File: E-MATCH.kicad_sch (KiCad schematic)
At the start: 7 parts, among them IC1 NCV81071BZR2G, J2 691137710002, Q1 IRF3205, U1 TMCS1108A2UQDR

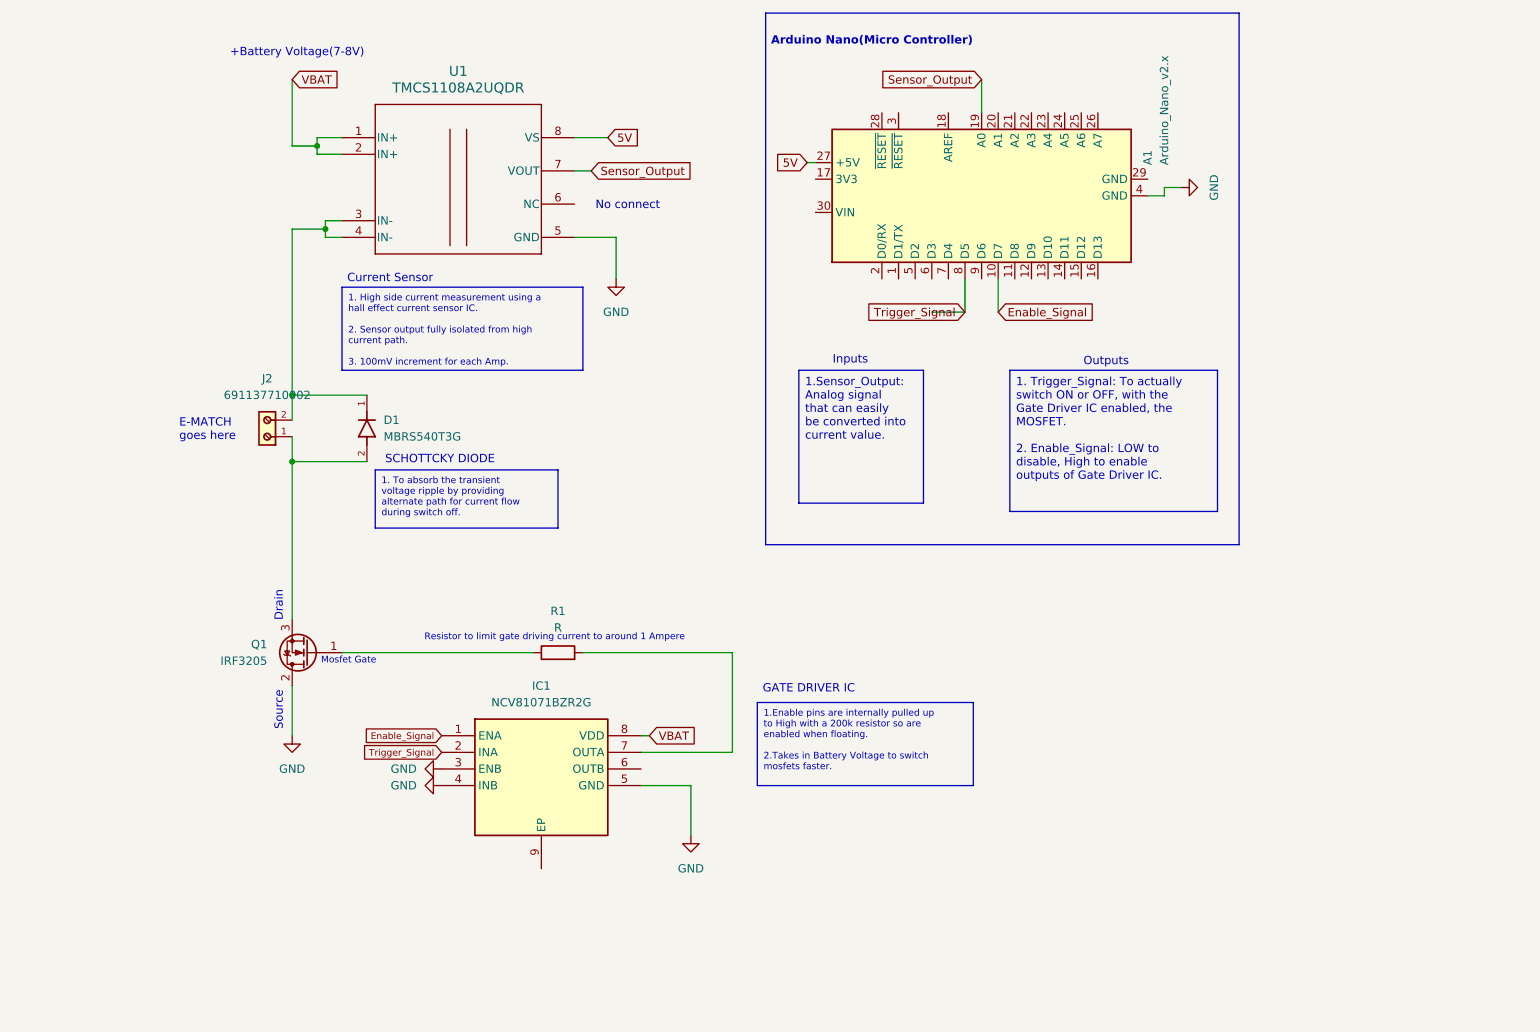
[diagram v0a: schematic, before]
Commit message: Neat placement for schematic
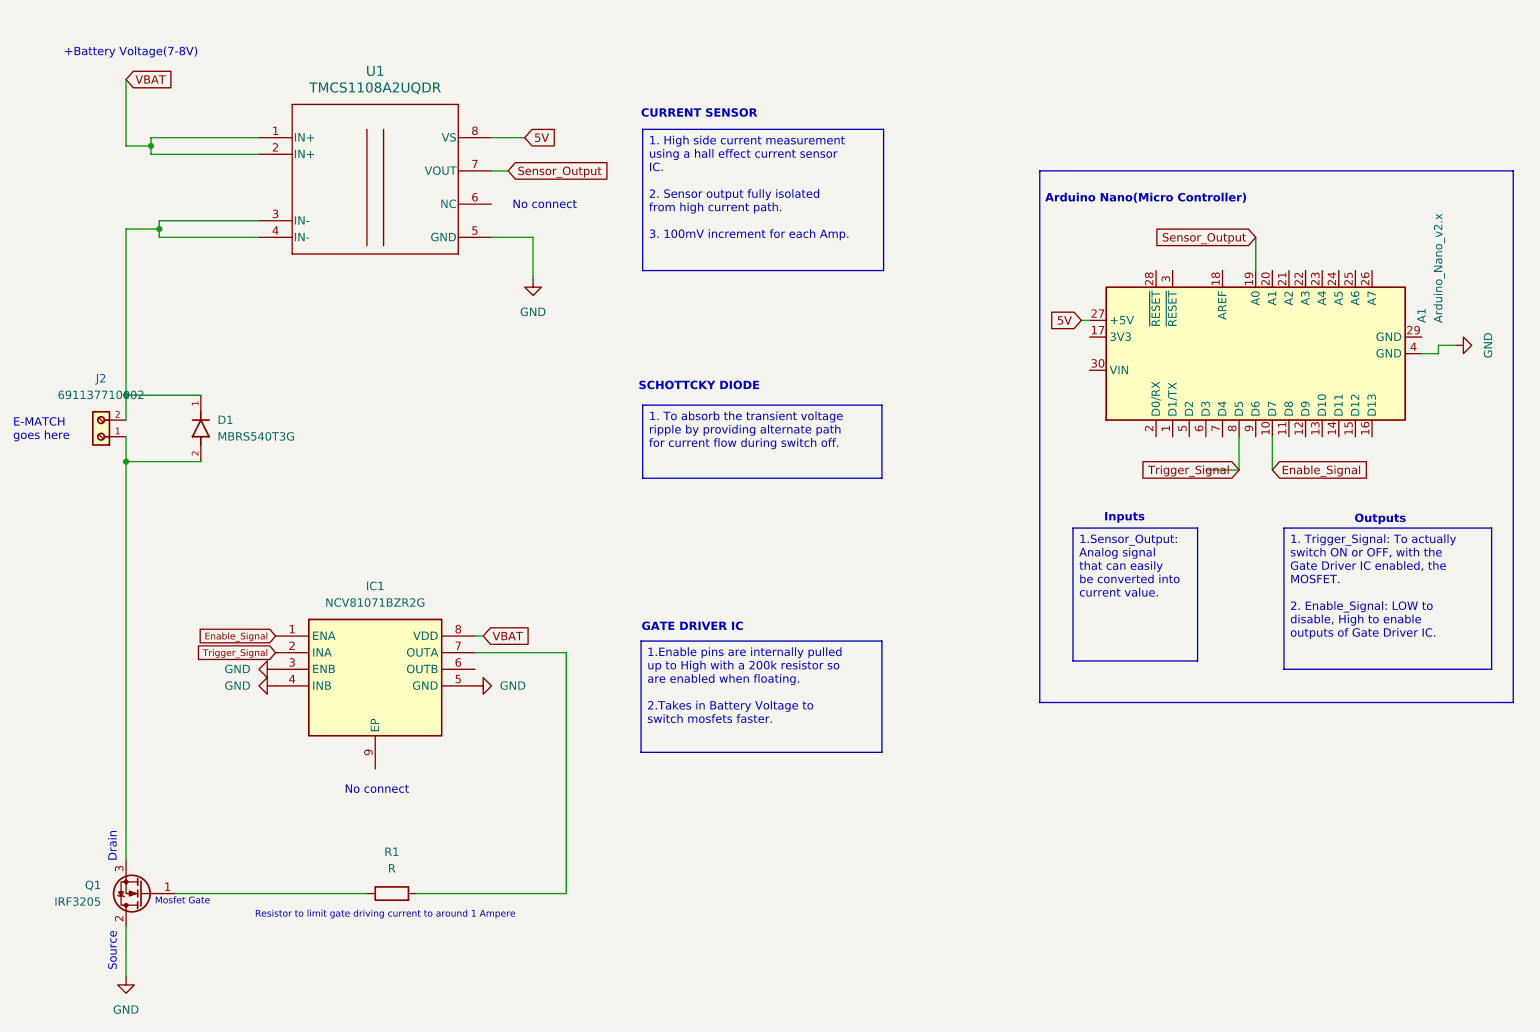
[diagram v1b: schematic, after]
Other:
- note added: "CURRENT SENSOR"
- note removed: "Current Sensor"
- moved on the sheet: A1, D1, IC1, J2, Q1, R1, U1
